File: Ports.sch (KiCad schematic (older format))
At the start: 5 parts, among them J5 Joystick_Port, J6 Joystick_Port

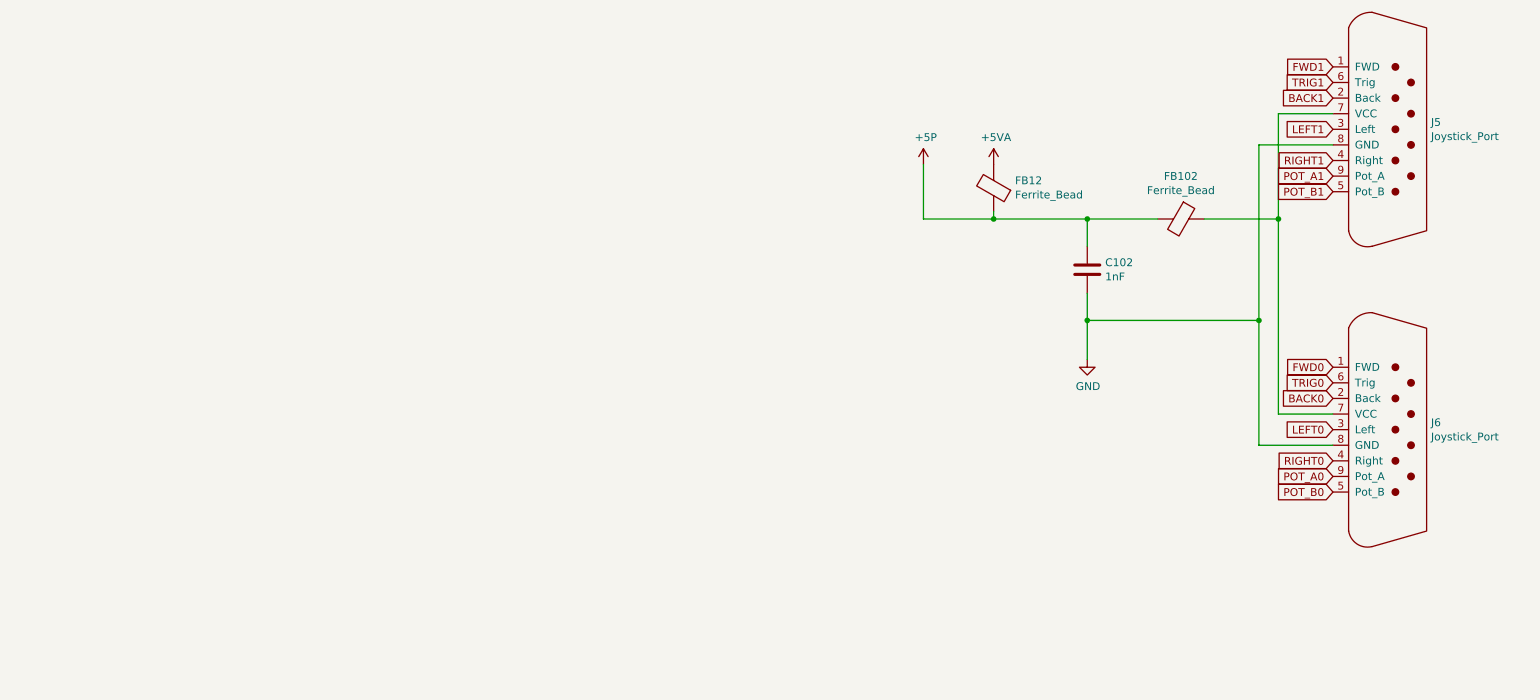
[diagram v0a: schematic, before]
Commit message: PIA and POKEY
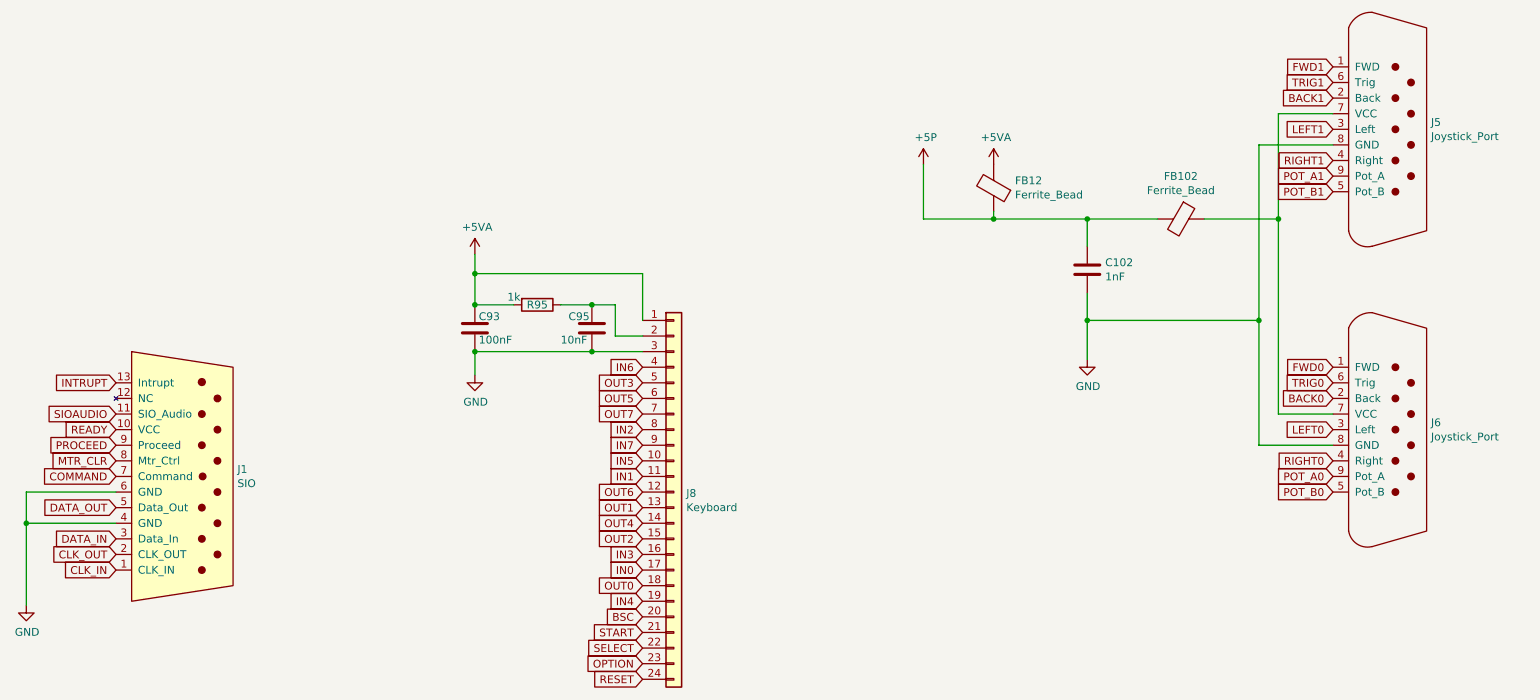
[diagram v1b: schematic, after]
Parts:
- added C93: 100nF, Atari:C_Axial_L5.1mm_D2.5mm_P12.50mm_Horizontal, symbol Device:C
- added C95: 10nF, Atari:C_Axial_L5.1mm_D2.5mm_P12.50mm_Horizontal, symbol Device:C
- added J1: SIO, Atari:SIO_Slot, symbol Atari:SIO_Port
- added J8: Keyboard, Connector_PinHeader_2.54mm:PinHeader_1x24_P2.54mm_Vertical, symbol Connector_Generic:Conn_01x24
- added R95: 1k, Atari:R_Axial_DIN0207_L3.6mm_D2.2mm_P10.16mm_Horizontal, symbol Device:R
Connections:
- net +5VA: now also C93.1, J8.1 (Pin_1), R95.2
- net GND: now also C93.2, C95.2, J1.4 (GND), J1.6 (GND), J8.3 (Pin_3)
- new net: C95.1, J8.2 (Pin_2), R95.1
- new net BSC: J8.20 (Pin_20)
- new net CLK_IN: J1.1 (CLK_IN)
- new net CLK_OUT: J1.2 (CLK_OUT)
- new net COMMAND: J1.7 (Command)
- new net DATA_IN: J1.3 (Data_In)
- new net DATA_OUT: J1.5 (Data_Out)
- new net IN0: J8.17 (Pin_17)
- new net IN1: J8.11 (Pin_11)
- new net IN2: J8.8 (Pin_8)
- new net IN3: J8.16 (Pin_16)
- new net IN4: J8.19 (Pin_19)
- new net IN5: J8.10 (Pin_10)
- new net IN6: J8.4 (Pin_4)
- new net IN7: J8.9 (Pin_9)
- new net INTRUPT: J1.13 (Intrupt)
- new net MTR_CLR: J1.8 (Mtr_Ctrl)
- new net OPTION: J8.23 (Pin_23)
- new net OUT0: J8.18 (Pin_18)
- new net OUT1: J8.13 (Pin_13)
- new net OUT2: J8.15 (Pin_15)
- new net OUT3: J8.5 (Pin_5)
- new net OUT4: J8.14 (Pin_14)
- new net OUT5: J8.6 (Pin_6)
- new net OUT6: J8.12 (Pin_12)
- new net OUT7: J8.7 (Pin_7)
- new net PROCEED: J1.9 (Proceed)
- new net READY: J1.10 (VCC)
- new net RESET: J8.24 (Pin_24)
- new net SELECT: J8.22 (Pin_22)
- new net SIOAUDIO: J1.11 (SIO_Audio)
- new net START: J8.21 (Pin_21)
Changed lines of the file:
@@
 	7025 2525 7025 2175
 Connection ~ 7475 2525
+$Comp
+L Atari:SIO_Port J1
+U 1 1 603D412B
+P 800 4175
+F 0 "J1" H 2628 4221 50  0000 L CNN
+F 1 "SIO" H 2628 4130 50  0000 L CNN
+F 2 "Atari:SIO_Slot" H 800 4175 50  0001 C CNN
+F 3 "" H 800 4175 50  0001 C CNN
+	1    800  4175
+	1    0    0    -1
+$EndComp
+Text GLabel 1850 4775 0    50   Input ~ 0
+CLK_IN
+Text GLabel 1850 4675 0    50   Input ~ 0
+CLK_OUT
+Text GLabel 1850 4575 0    50   Input ~ 0
+DATA_IN
+Text GLabel 1850 4375 0    50   Input ~ 0
+DATA_OUT
+Text GLabel 1850 4175 0    50   Input ~ 0
+COMMAND
+Text GLabel 1850 4075 0    50   Input ~ 0
+MTR_CLR
+Text GLabel 1850 3975 0    50   Input ~ 0
+PROCEED
+Text GLabel 1850 3775 0    50   Input ~ 0
+SIOAUDIO
+Text GLabel 1850 3575 0    50   Input ~ 0
+INTRUPT
+Wire Wire Line
+	1850 4275 1275 4275
+Wire Wire Line
+	1275 4275 1275 4475
+Wire Wire Line
+	1275 4475 1850 4475
+$Comp
+L power:GND #PWR0217
+U 1 1 603D6D5A
+P 1275 5000
+F 0 "#PWR0217" H 1275 4750 50  0001 C CNN
+F 1 "GND" H 1280 4827 50  0000 C CNN
+F 2 "" H 1275 5000 50  0001 C CNN
+F 3 "" H 1275 5000 50  0001 C CNN
+	1    1275 5000
+	1    0    0    -1
+$EndComp
+Wire Wire Line
+	1275 4475 1275 5000
+Connection ~ 1275 4475
+Text GLabel 1850 3875 0    50   Input ~ 0
+READY
+$Comp
+L Connector_Generic:Conn_01x24 J8
+U 1 1 603E550F
+P 5425 4275
+F 0 "J8" H 5505 4267 50  0000 L CNN
+F 1 "Keyboard" H 5505 4176 50  0000 L CNN
+F 2 "Connector_PinHeader_2.54mm:PinHeader_1x24_P2.54mm_Vertical" H 5425 4275 50  0001 C CNN
+F 3 "~" H 5425 4275 50  0001 C CNN
+	1    5425 4275
+	1    0    0    -1
+$EndComp
+Text GLabel 5225 5475 0    50   Input ~ 0
+RESET
+Text GLabel 5225 5375 0    50   Input ~ 0
+OPTION
+Text GLabel 5225 5275 0    50   Input ~ 0
+SELECT
+Text GLabel 5225 5175 0    50   Input ~ 0
+START
+Text GLabel 5225 5075 0    50   Input ~ 0
+BSC
+Text GLabel 5225 4975 0    50   Input ~ 0
+IN4
+Text GLabel 5225 4875 0    50   Input ~ 0
+OUT0
+Text GLabel 5225 4775 0    50   Input ~ 0
+IN0
+Text GLabel 5225 4675 0    50   Input ~ 0
+IN3
+Text GLabel 5225 4575 0    50   Input ~ 0
+OUT2
+Text GLabel 5225 4475 0    50   Input ~ 0
+OUT4
+Text GLabel 5225 4375 0    50   Input ~ 0
+OUT1
+Text GLabel 5225 4275 0    50   Input ~ 0
+OUT6
+Text GLabel 5225 4175 0    50   Input ~ 0
+IN1
+Text GLabel 5225 4075 0    50   Input ~ 0
+IN5
+Text GLabel 5225 3975 0    50   Input ~ 0
+IN7
+Text GLabel 5225 3875 0    50   Input ~ 0
+IN2
+Text GLabel 5225 3775 0    50   Input ~ 0
+OUT7
+Text GLabel 5225 3675 0    50   Input ~ 0
+OUT5
+Text GLabel 5225 3575 0    50   Input ~ 0
+OUT3
+Text GLabel 5225 3475 0    50   Input ~ 0
+IN6
+$Comp
+L power:GND #PWR0218
+U 1 1 603EA252
+P 4150 3525
+F 0 "#PWR0218" H 4150 3275 50  0001 C CNN
+F 1 "GND" H 4155 3352 50  0000 C CNN
+F 2 "" H 4150 3525 50  0001 C CNN
+F 3 "" H 4150 3525 50  0001 C CNN
+	1    4150 3525
+	1    0    0    -1
+$EndComp
+Wire Wire Line
+	4150 3375 4150 3525
+$Comp
+L Device:R R95
+U 1 1 603EACD2
+P 4550 3075
+F 0 "R95" V 4550 3075 50  0000 C CNN
+F 1 "1k" V 4500 2925 50  0000 C CNN
+F 2 "Atari:R_Axial_DIN0207_L3.6mm_D2.2mm_P10.16mm_Horizontal" V 4480 3075 50  0001 C CNN
+F 3 "~" H 4550 3075 50  0001 C CNN
+	1    4550 3075
+	0    1    1    0
+$EndComp
+$Comp
+L Device:C C93
+U 1 1 603EB979
+P 4150 3225
+F 0 "C93" H 4175 3300 50  0000 L CNN
+F 1 "100nF" H 4175 3150 50  0000 L CNN
+F 2 "Atari:C_Axial_L5.1mm_D2.5mm_P12.50mm_Horizontal" H 4188 3075 50  0001 C CNN
+F 3 "~" H 4150 3225 50  0001 C CNN
+	1    4150 3225
+	1    0    0    -1
+$EndComp
+Connection ~ 4150 3375
+Wire Wire Line
+	4150 3375 4900 3375
+$Comp
+L Device:C C95
+U 1 1 603ECF87
+P 4900 3225
+F 0 "C95" H 4750 3300 50  0000 L CNN
+F 1 "10nF" H 4700 3150 50  0000 L CNN
+F 2 "Atari:C_Axial_L5.1mm_D2.5mm_P12.50mm_Horizontal" H 4938 3075 50  0001 C CNN
+F 3 "~" H 4900 3225 50  0001 C CNN
+	1    4900 3225
+	1    0    0    -1
+$EndComp
+Connection ~ 4900 3375
+Wire Wire Line
+	4900 3375 5225 3375
+Wire Wire Line
+	4700 3075 4900 3075
+Wire Wire Line
+	4150 3075 4400 3075
+Wire Wire Line
+	5225 3275 5050 3275
+Wire Wire Line
+	5050 3275 5050 3075
+Wire Wire Line
+	5050 3075 4900 3075
+Connection ~ 4900 3075
+Wire Wire Line
+	5225 3175 5225 2875
+Wire Wire Line
+	5225 2875 4150 2875
+Wire Wire Line
+	4150 2875 4150 3075
+Connection ~ 4150 3075
+$Comp
+L power:+5VA #PWR0219
+U 1 1 603EF951
+P 4150 2750
+F 0 "#PWR0219" H 4150 2600 50  0001 C CNN
+F 1 "+5VA" H 4165 2923 50  0000 C CNN
+F 2 "" H 4150 2750 50  0001 C CNN
+F 3 "" H 4150 2750 50  0001 C CNN
+	1    4150 2750
+	1    0    0    -1
+$EndComp
+Wire Wire Line
+	4150 2750 4150 2875
+Connection ~ 4150 2875
 $EndSCHEMATC
